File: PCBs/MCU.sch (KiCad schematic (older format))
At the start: 20 parts, among them CON2 AVR-ISP-6, J10 SPK, J7 Conn_01x10, U6 ATMEGA328P-AU, Y2 16Mhz

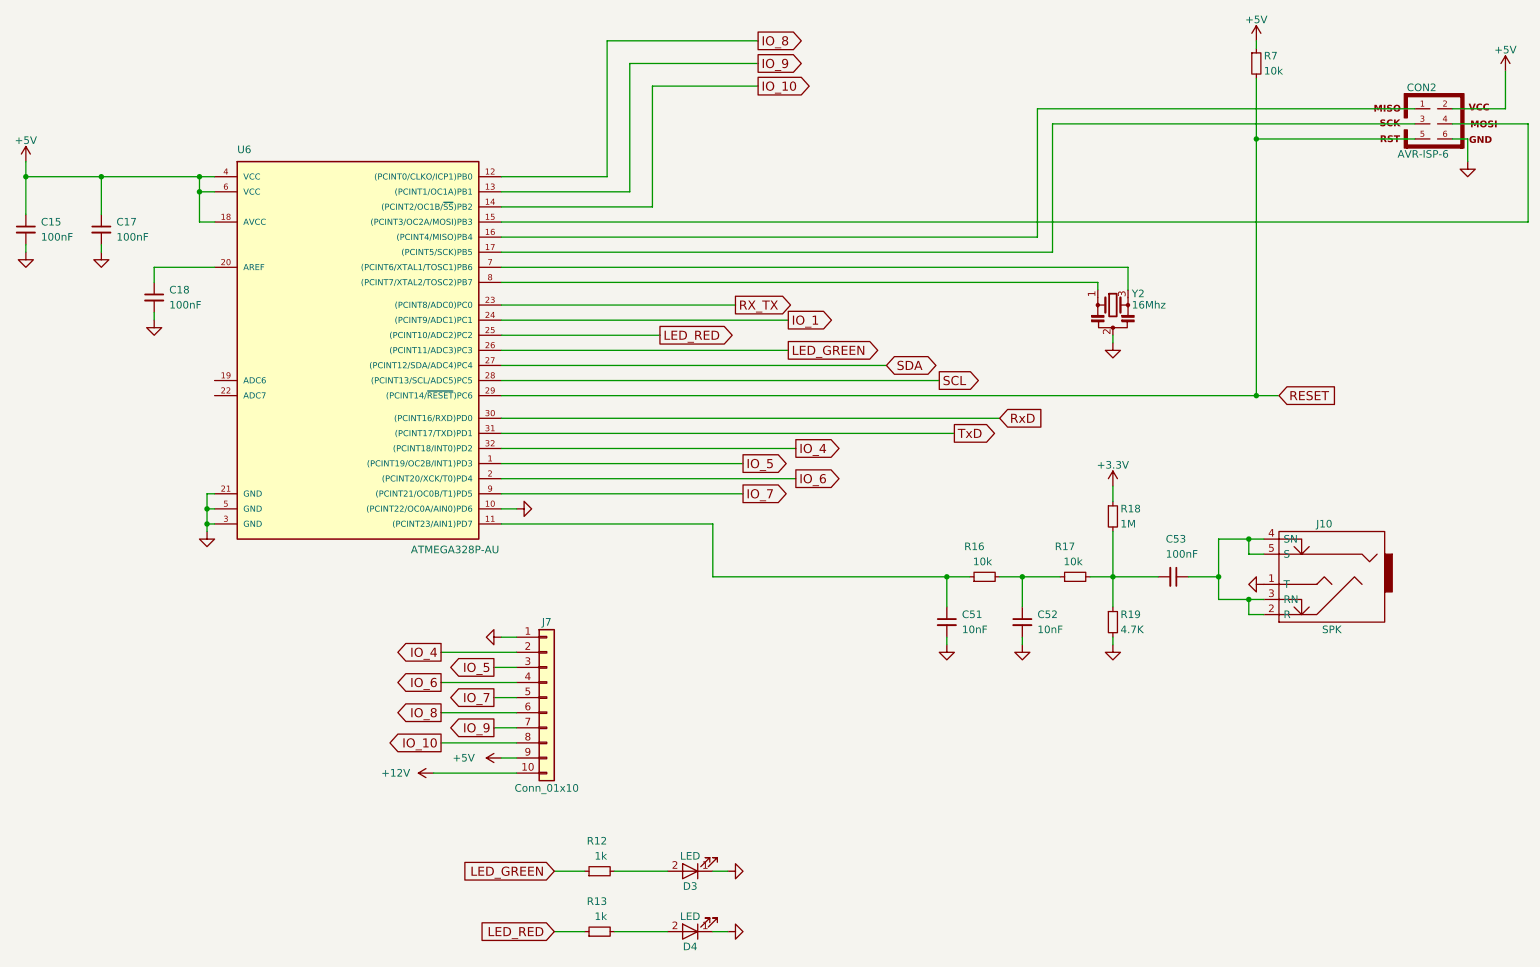
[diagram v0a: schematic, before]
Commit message: INIT project, si5351 generate properly frequency
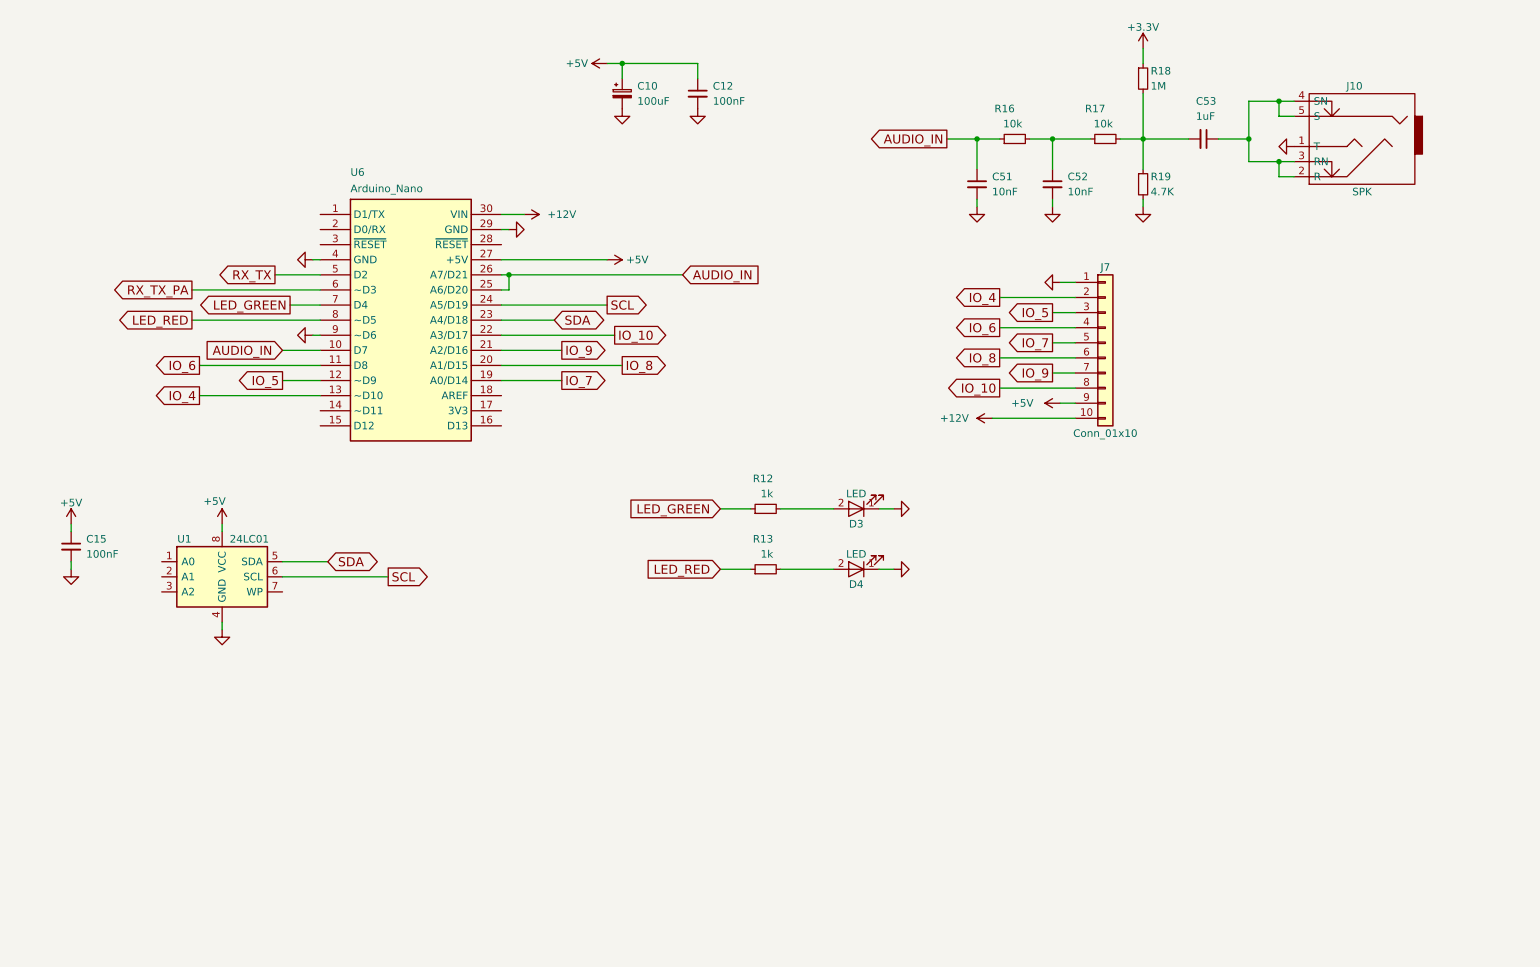
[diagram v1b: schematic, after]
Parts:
- removed C17, C18: 100nF, LCSDR:C_1206_0603, symbol C_Small
- removed CON2: AVR-ISP-6, Connectors_IDC:IDC-Header_2x03_Pitch2.54mm_Straight, symbol AVR-ISP-6
- removed R7: 10k, LCSDR:R_1206_0603, symbol R_Small
- removed U6: ATMEGA328P-AU, Housings_QFP:TQFP-32_7x7mm_Pitch0.8mm, symbol ATMEGA328P-AU
- removed Y2: 16Mhz, LCSDR:Crystal_SMD_3213_3.2x1.3mm, symbol Resonator_Small
- added C10: 100uF, Capacitors_THT:CP_Radial_D6.3mm_P2.50mm, symbol CP_Small
- added C12: 100nF, Capacitors_SMD:C_0603_HandSoldering, symbol C_Small
- added U1: 24LC01, Housings_SOIC:SOIC-8_3.9x4.9mm_Pitch1.27mm, symbol 24LC01
- added U6: Arduino_Nano, Arduino:Arduino_Nano, symbol Arduino_Nano
- C15, C51, C52: footprint LCSDR:C_1206_0603 -> Capacitors_SMD:C_0603_HandSoldering
- C53: value 100nF -> 1uF; footprint LCSDR:C_1206_0603 -> Capacitors_SMD:C_0603_HandSoldering
- D3, D4: footprint LEDs:LED_D3.0mm_Horizontal_O3.81mm_Z10.0mm -> LEDs:LED_0603_HandSoldering
- R12, R13, R16, R17, R18, R19: footprint LCSDR:R_1206_0603 -> Resistors_SMD:R_0603_HandSoldering
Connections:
- net +12V: now also U6.30 (VIN)
- net +5V: now also C10.1, C12.1, U1.8 (VCC), U6.27 (+5V)
- net GND: now also C10.2, C12.2, U1.4 (GND), U6.29 (GND), U6.4 (GND), U6.9 (~~D6)
- net IO_10: now also U6.22 (A3/D17)
- net IO_4: now also U6.13 (~~D10)
- net IO_5: now also U6.12 (~~D9)
- net IO_6: now also U6.11 (D8)
- net IO_7: now also U6.19 (A0/D14)
- net IO_8: now also U6.20 (A1/D15)
- net IO_9: now also U6.21 (A2/D16)
- net LED_GREEN: now also U6.7 (D4)
- net LED_RED: now also U6.8 (~~D5)
- net RX_TX: now also U6.5 (D2)
- net SCL: now also U1.6 (SCL), U6.24 (A5/D19)
- net SDA: now also U1.5 (SDA), U6.23 (A4/D18)
- net AUDIO_IN: now reaches C51.1, R16.1
- net AUDIO_IN: now also U6.10 (D7), U6.25 (A6/D20), U6.26 (A7/D21)
- new net RX_TX_PA: U6.6 (~~D3)
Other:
- moved on the sheet: C15, C51, C52, C53, D3, D4, J10, J7, R12, R13, R16, R17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
